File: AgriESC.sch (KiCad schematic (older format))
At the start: 128 parts, among them J1 SUPPLY, J10 GPIO, J11 USB_OTG, J12 HALL_ENC, J2 PH_A, J3 PH_B, J4 PH_C, J6 COMM, J7 SERVO, J8 CAN, J9 SWD, SW1 SW_SPDT, U1 FDMS7698, U10 STM32F405RGT6, U11 DRV8303, U12 TJA1051TK-3, U13 LMR16006YQ, U14 MCP1700-3302E_SOT23, U15 MCP1700-3302E_SOT23, U2 FDMS7698, U3 FDMS7698, U4 FDMS7698, U5 FDMS7698, U6 FDMS7698, U7 MAX9920, U8 MAX9920, U9 MAX9920, Y1 8M Resonator

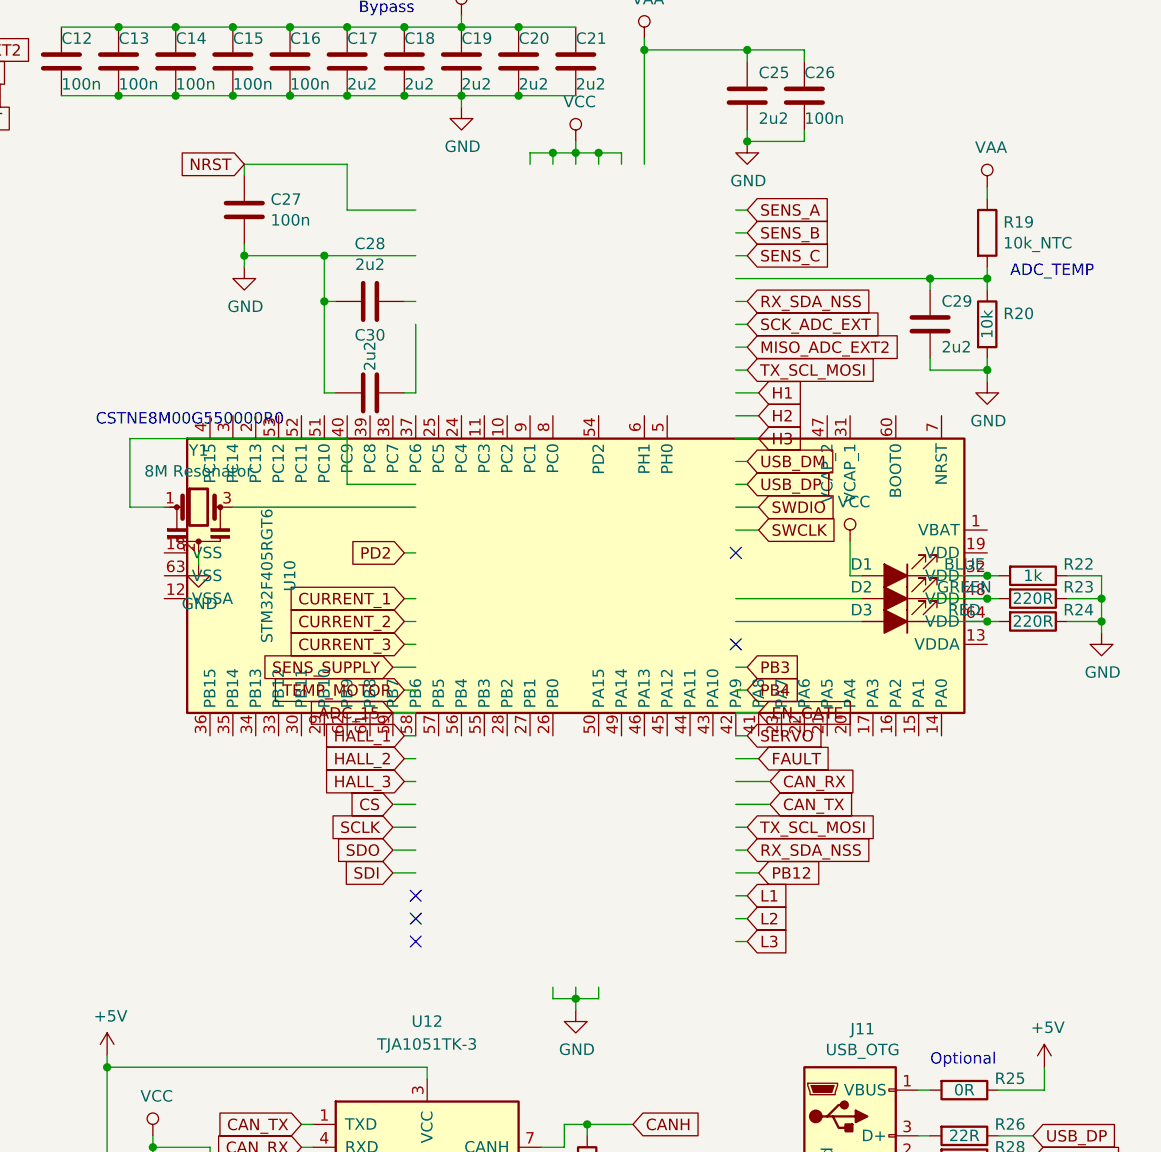
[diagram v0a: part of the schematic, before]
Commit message: Fix to schematic
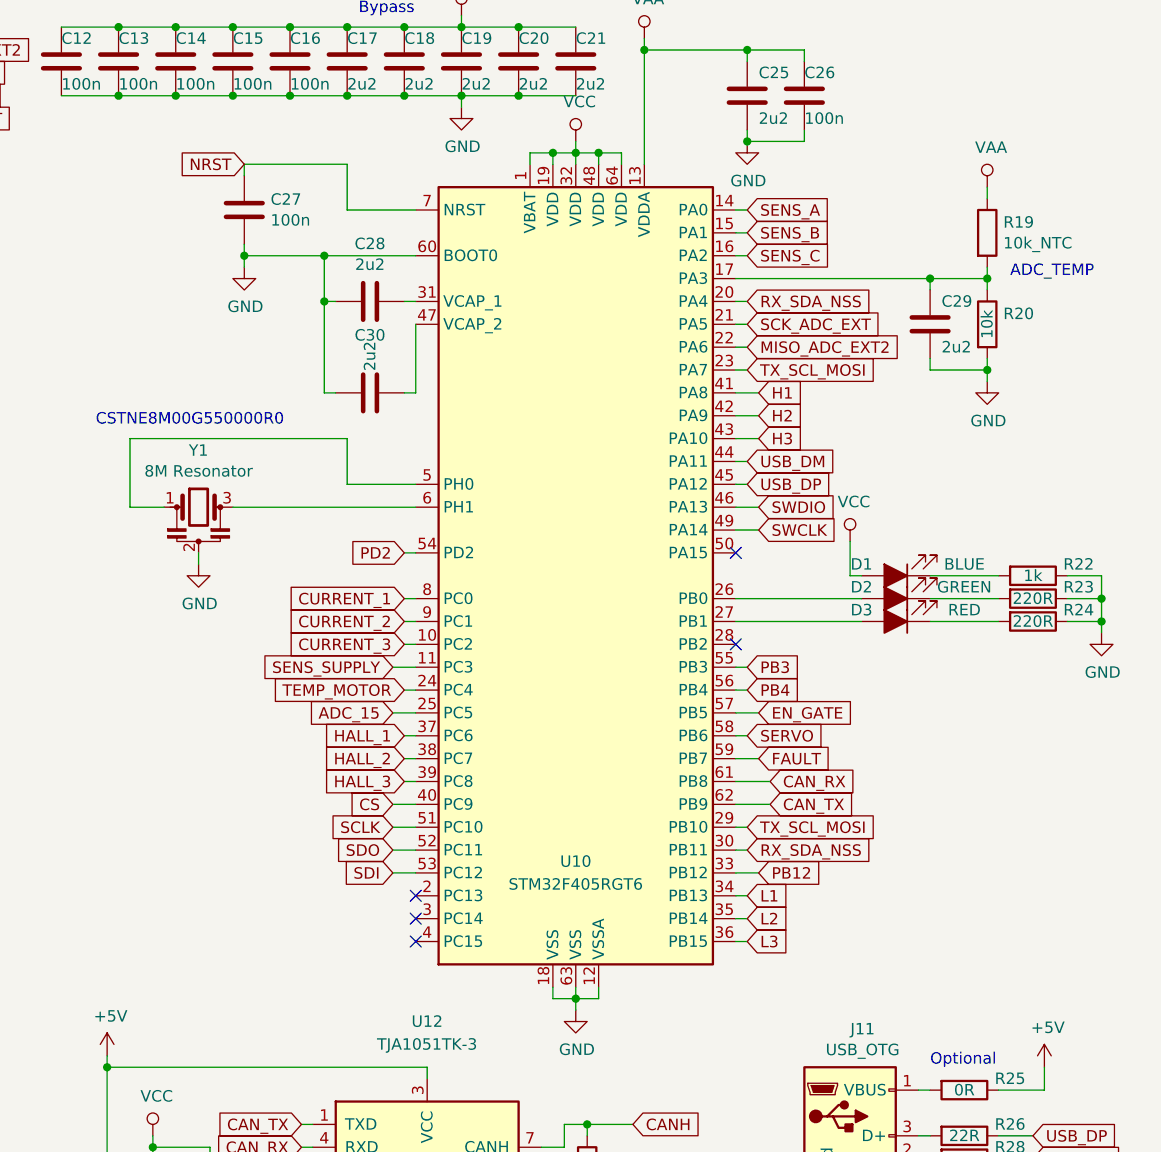
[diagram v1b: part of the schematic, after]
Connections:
- wire segments 600 -> 597
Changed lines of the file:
@@
 F 3 "http://www.st.com/st-web-ui/static/active/en/resource/technical/document/datasheet/DM00037051.pdf" H 8650 3200 50  0001 C CNN
 	1    8650 3200
-	0    1    1    0
+	1    0    0    -1
 $EndComp
 Wire Wire Line
@@
 	9450 2400 9350 2400
 Wire Wire Line
-	9350 2500 9450 2500
-Wire Wire Line
 	9350 2600 9450 2600
 Text GLabel 9400 2700 2    50   Input ~ 0
@@
 	7950 2000 7900 2000
 Wire Wire Line
-	7950 2100 7950 2400
-Wire Wire Line
 	7950 2400 7900 2400
 Wire Wire Line
@@
 	9850 3200 9900 3200
 Wire Wire Line
-	10500 3200 10450 3200
-Wire Wire Line
 	9350 3300 9900 3300
 Wire Wire Line
@@
 $EndComp
 Wire Wire Line
-	10500 3300 10450 3300
-Wire Wire Line
-	10200 3400 10450 3400
-Wire Wire Line
 	10800 3200 10950 3200
 Wire Wire Line
@@
 Wire Wire Line
 	7000 3100 7000 3150
-Connection ~ 10450 3200
 Wire Wire Line
-	10450 3200 10200 3200
-Connection ~ 10450 3300
+	9350 2500 9450 2500
+Wire Wire Line
+	7950 2100 7950 2400
+Wire Wire Line
+	10200 3400 10500 3400
 Wire Wire Line
-	10450 3300 10200 3300
-Connection ~ 10450 3400
+	10200 3300 10500 3300
 Wire Wire Line
-	10450 3400 10500 3400
+	10200 3200 10500 3200
 $EndSCHEMATC

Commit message: Before CAN package update
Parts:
- U12: footprint Package_DFN_QFN:DFN-8-1EP_3x3mm_P0.65mm_EP1.55x2.4mm -> Housings_DFN_QFN:DFN-8-1EP_3x3mm_Pitch0.65mm
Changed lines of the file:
@@
 EESchema Schematic File Version 4
 LIBS:AgriESC-cache
-EELAYER 26 0
+EELAYER 29 0
 EELAYER END
 $Descr A4 11693 8268
@@
 F 0 "U12" H 8000 6450 50  0000 C CNN
 F 1 "TJA1051TK-3" H 8000 6350 50  0000 C CNN
-F 2 "Package_DFN_QFN:DFN-8-1EP_3x3mm_P0.65mm_EP1.55x2.4mm" H 8000 5300 50  0001 C CIN
+F 2 "Housings_DFN_QFN:DFN-8-1EP_3x3mm_Pitch0.65mm" H 8000 5300 50  0001 C CIN
 F 3 "http://www.nxp.com/documents/data_sheet/TJA1051.pdf" H 8000 5800 50  0001 C CNN
 	1    8000 5800
